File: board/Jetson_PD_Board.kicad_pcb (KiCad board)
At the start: 2 copper layers, 42.6 x 35.8 mm, 47 parts, among them J1 USB4081-03-A, J2 768250002, Q1 NTTFS5C673NLTAG, Q2 NTTFS5C673NLTAG, Q3 NTTFS5C673NLTAG, U1 APK43070DKZ-13-FA01, U2 USBLC6-2SC6

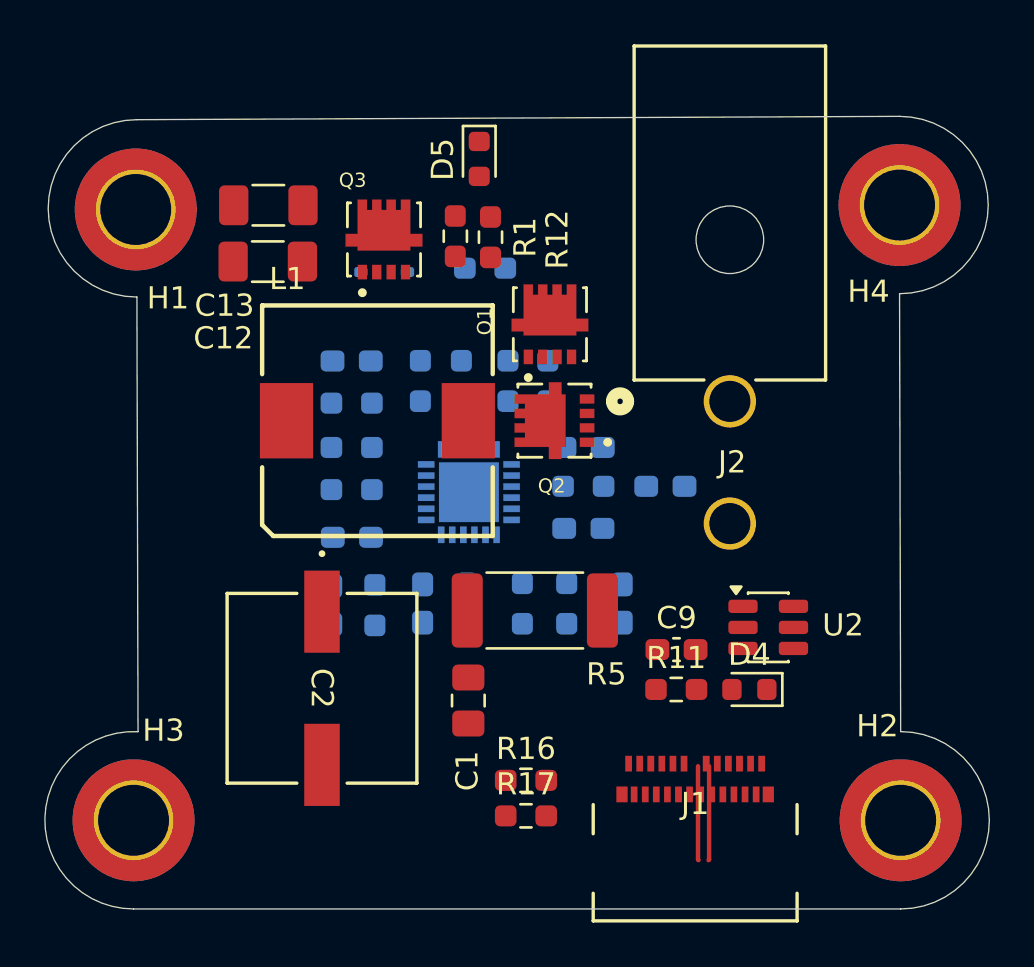
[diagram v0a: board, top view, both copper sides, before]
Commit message: Adjusted grid
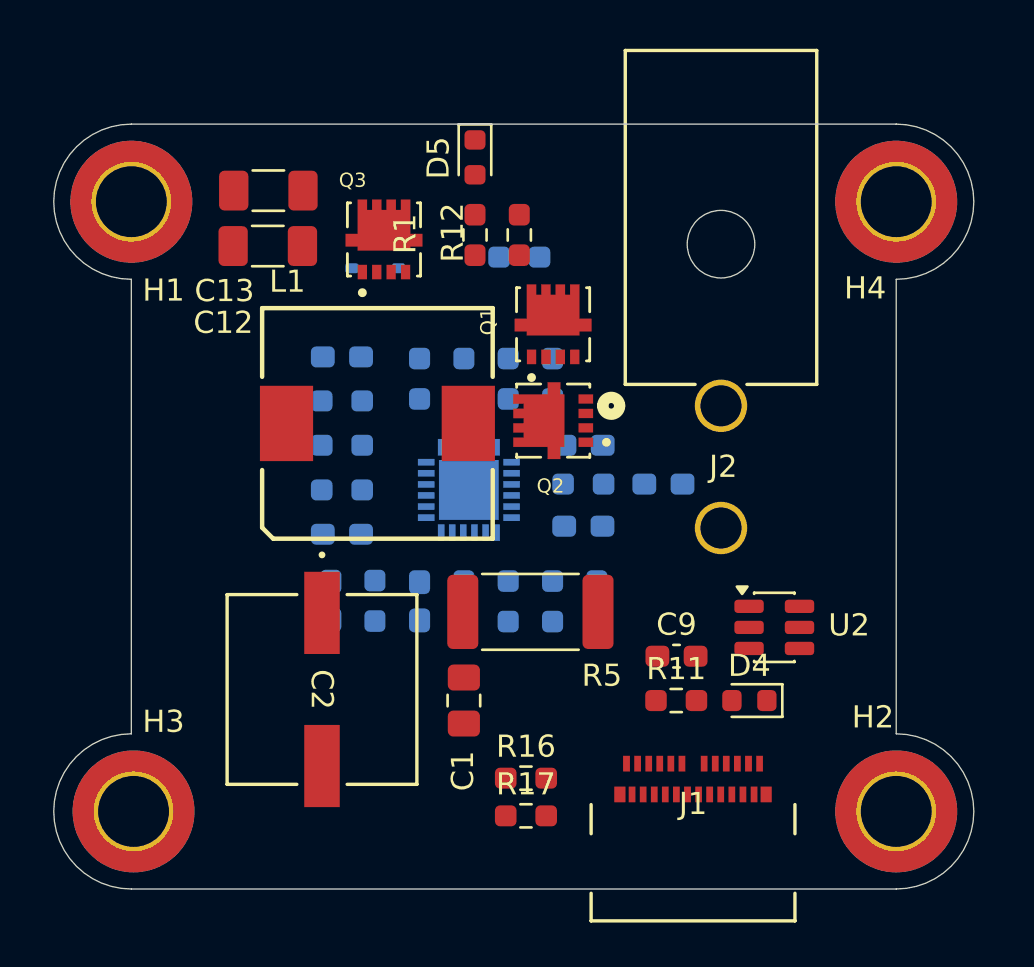
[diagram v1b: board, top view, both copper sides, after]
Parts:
- moved R13 1.62 mm to (122.5, 86.5)
- moved R12 1.30 mm to (122.5, 85.5), turned to -90 degrees
- moved C7 1.14 mm to (126.0, 102.0)
- moved R1 0.89 mm to (120.5, 85.5), turned to -90 degrees
- moved C12 0.70 mm to (111.2, 86.0)
- moved C13 0.66 mm to (111.2, 83.5)
- moved R6 0.65 mm to (122.0, 102.0)
- moved R7 0.65 mm to (124.0, 102.0)
- moved D4 0.50 mm to (132.9, 106.5)
- moved R11 0.50 mm to (129.6, 106.5)
- moved C11 0.47 mm to (114.5, 91.0)
- moved C14 0.47 mm to (114.5, 99.0)
- moved R14 0.45 mm to (114.5, 95.0)
- moved TH1 0.45 mm to (114.5, 93.0)
- moved H2 0.45 mm to (139.5, 111.5)
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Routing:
- net CC2: track 4.25 -> 0.00 mm
- net /USB_DP: track 4.25 -> 0.00 mm
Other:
- board size 42.6 x 35.8 mm -> 41.5 x 34.5 mm
